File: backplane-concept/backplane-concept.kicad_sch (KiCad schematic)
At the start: 2 parts

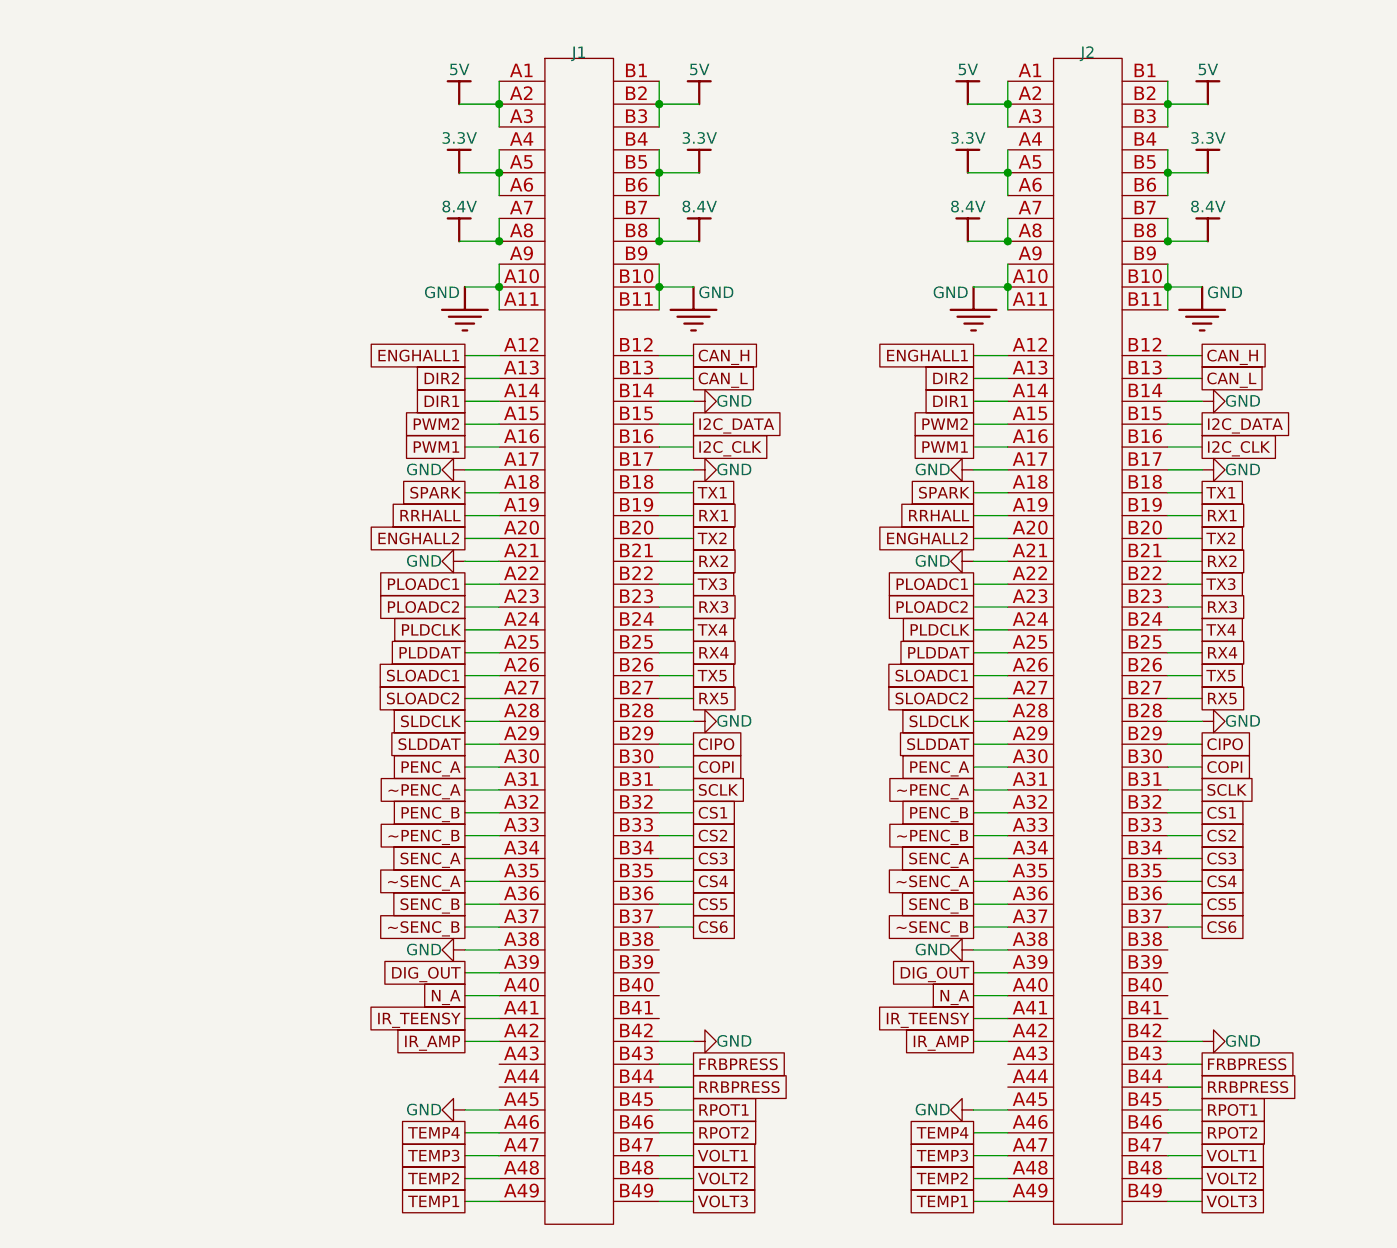
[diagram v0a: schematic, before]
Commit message: Rev
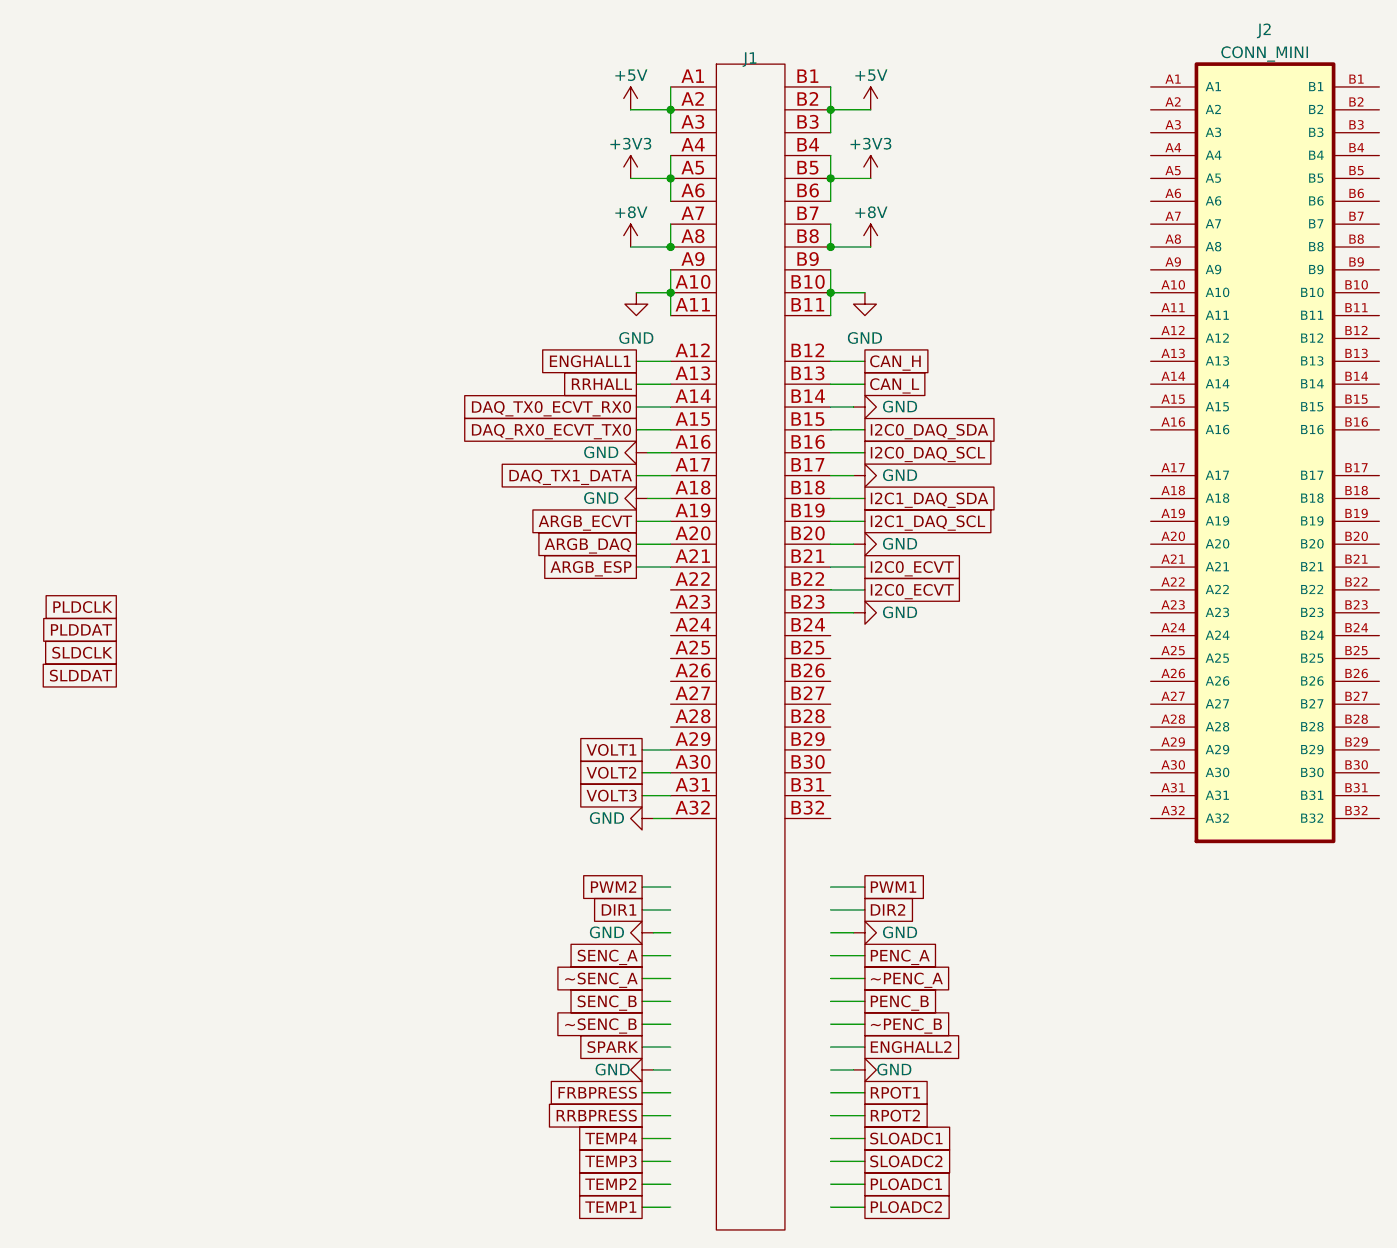
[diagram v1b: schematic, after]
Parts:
- removed J2: ~, !footprints:9-1734774-5, symbol 9-1734774-5:PCIE
- added J2: CONN_MINI, CONN_10018784-10201TLF, symbol 10018784-10201TLF:10018784-10201TLF
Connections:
- net RX3 is gone; now on net GND: J1.B23
- net TX2 is gone; now on net GND: J1.B20
- net TX3 is gone; now on net I2C0_ECVT: J1.B22
- net DIR1: no longer J1.A14
- net DIR2: no longer J1.A13
- net ENGHALL2: no longer J1.A20
- net FRBPRESS: no longer J1.B43
- net GND: now also J1.A16, J1.A18, J1.A32; no longer J1.A17, J1.A21, J1.A38, J1.A45, J1.B28, J1.B42
- net PENC_A: no longer J1.A30
- net PENC_B: no longer J1.A32
- net PLDCLK: no longer J1.A24
- net PLDDAT: no longer J1.A25
- net PLOADC1: no longer J1.A22
- net PLOADC2: no longer J1.A23
- net PWM1: no longer J1.A16
- net PWM2: no longer J1.A15
- net RPOT1: no longer J1.B45
- net RPOT2: no longer J1.B46
- net RRBPRESS: no longer J1.B44
- net RRHALL: now also J1.A13; no longer J1.A19
- net SENC_A: no longer J1.A34
- net SENC_B: no longer J1.A36
- net SLDCLK: no longer J1.A28
- net SLDDAT: no longer J1.A29
- net SLOADC1: no longer J1.A26
- net SLOADC2: no longer J1.A27
- net SPARK: no longer J1.A18
- net TEMP1: no longer J1.A49
- net TEMP2: no longer J1.A48
- net TEMP3: no longer J1.A47
- net TEMP4: no longer J1.A46
- net VOLT1: now also J1.A29; no longer J1.B47
- net VOLT2: now also J1.A30; no longer J1.B48
- net VOLT3: now also J1.A31; no longer J1.B49
- net ~PENC_A: no longer J1.A31
- net ~PENC_B: no longer J1.A33
- net ~SENC_A: no longer J1.A35
- net ~SENC_B: no longer J1.A37
- net 3.3V renamed +3V3
- net 5V renamed +5V
- net 8.4V renamed +8V
- net CIPO: no longer names the net of J1.B29
- net COPI: no longer names the net of J1.B30
- net CS1: no longer names the net of J1.B32
- removed net CS2: J1.B33
- removed net CS3: J1.B34
- removed net CS4: J1.B35
- removed net CS5: J1.B36
- removed net CS6: J1.B37
- removed net DIG_OUT: J1.A39
- net I2C_CLK renamed I2C0_DAQ_SCL
- net I2C_DATA renamed I2C0_DAQ_SDA
- removed net IR_AMP: J1.A42
- removed net IR_TEENSY: J1.A41
- removed net N_A: J1.A40
- net RX1 renamed I2C1_DAQ_SCL
- net RX2 renamed I2C0_ECVT
- net RX4: no longer names the net of J1.B25
- net RX5: no longer names the net of J1.B27
- net SCLK: no longer names the net of J1.B31
- net TX1 renamed I2C1_DAQ_SDA
- net TX4: no longer names the net of J1.B24
- net TX5: no longer names the net of J1.B26
- new net ARGB_DAQ: J1.A20
- new net ARGB_ECVT: J1.A19
- new net ARGB_ESP: J1.A21
- new net DAQ_RX0_ECVT_TX0: J1.A15
- new net DAQ_TX0_ECVT_RX0: J1.A14
- new net DAQ_TX1_DATA: J1.A17

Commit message: Backplane Ideas
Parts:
- removed J1: ~, !footprints:9-1734774-5, symbol 9-1734774-5:PCIE
- removed J2: CONN_MINI, CONN_10018784-10201TLF, symbol 10018784-10201TLF:10018784-10201TLF
- added J1: 6473427-1, 64734271, symbol 6473427-1:6473427-1
- added J2, J3, J4: PCIE_8x_Labeled, !footprints:9-1734774-5, symbol !CUSTOM:PCIE_8x_Labeled
- added J5, J6, J7, J8: CONN_MINI, !footprints:10018784-10200TLF, symbol !CUSTOM:PCIE_2x_Labeled
- added U4: ATA6561-GBQW-N, VDFN8_3X3_MCH, symbol ATA6561:ATA6561-GBQW-N
- added U5: ESP32-PICO-D4, Package_DFN_QFN:QFN-48-1EP_7x7mm_P0.5mm_EP5.3x5.3mm, symbol RF_Module:ESP32-PICO-D4
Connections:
- net +3V3: now also J1.B10, J1.B25, J1.B26, J2.A4 (+3V3), J2.A5 (+3V3), J2.A6 (+3V3), J2.B4 (+3V3), J2.B5 (+3V3), J2.B6 (+3V3), J3.A4 (+3V3), J3.A5 (+3V3), J3.A6 (+3V3), J3.B4 (+3V3), J3.B5 (+3V3), J3.B6 (+3V3), J4.A4 (+3V3), J4.A5 (+3V3), J4.A6 (+3V3), J4.B4 (+3V3), J4.B5 (+3V3), J4.B6 (+3V3), J5.A4 (+3V3), J5.A5 (+3V3), J5.A6 (+3V3), J5.B4 (+3V3), J5.B5 (+3V3), J5.B6 (+3V3), J6.A4 (+3V3), J6.A5 (+3V3), J6.A6 (+3V3), J6.B4 (+3V3), J6.B5 (+3V3), J6.B6 (+3V3), J7.A4 (+3V3), J7.A5 (+3V3), J7.A6 (+3V3), J7.B4 (+3V3), J7.B5 (+3V3), J7.B6 (+3V3), J8.A4 (+3V3), J8.A5 (+3V3), J8.A6 (+3V3), J8.B4 (+3V3), J8.B5 (+3V3), J8.B6 (+3V3)
- net +5V: now also J1.A1, J1.A10, J1.A18, J1.A26, J2.A1 (+5V), J2.A2 (+5V), J2.A3 (+5V), J2.B1 (+5V), J2.B2 (+5V), J2.B3 (+5V), J3.A1 (+5V), J3.A2 (+5V), J3.A3 (+5V), J3.B1 (+5V), J3.B2 (+5V), J3.B3 (+5V), J4.A1 (+5V), J4.A2 (+5V), J4.A3 (+5V), J4.B1 (+5V), J4.B2 (+5V), J4.B3 (+5V), J5.A1 (+5V), J5.A2 (+5V), J5.A3 (+5V), J5.B1 (+5V), J5.B2 (+5V), J5.B3 (+5V), J6.A1 (+5V), J6.A2 (+5V), J6.A3 (+5V), J6.B1 (+5V), J6.B2 (+5V), J6.B3 (+5V), J7.A1 (+5V), J7.A2 (+5V), J7.A3 (+5V), J7.B1 (+5V), J7.B2 (+5V), J7.B3 (+5V), J8.A1 (+5V), J8.A2 (+5V), J8.A3 (+5V), J8.B1 (+5V), J8.B2 (+5V), J8.B3 (+5V)
- net +8V: now also J1.B5, J1.B6, J2.A7 (VBATT), J2.A8 (VBATT), J2.B7 (VBATT), J2.B8 (VBATT), J3.A7 (VBATT), J3.A8 (VBATT), J3.B7 (VBATT), J3.B8 (VBATT), J4.A7 (VBATT), J4.A8 (VBATT), J4.B7 (VBATT), J4.B8 (VBATT), J5.A7 (VBATT), J5.A8 (VBATT), J5.B7 (VBATT), J5.B8 (VBATT), J6.A7 (VBATT), J6.A8 (VBATT), J6.B7 (VBATT), J6.B8 (VBATT), J7.A7 (VBATT), J7.A8 (VBATT), J7.B7 (VBATT), J7.B8 (VBATT), J8.A7 (VBATT), J8.A8 (VBATT), J8.B7 (VBATT), J8.B8 (VBATT)
- net CAN_H: now also J2.B12 (CAN_H), J3.B12 (CAN_H), J4.B12 (CAN_H), J5.B12 (CAN_H), J6.B12 (CAN_H), J7.B12 (CAN_H), J8.B12 (CAN_H)
- net CAN_L: now also J2.B13 (CAN_L), J3.B13 (CAN_L), J4.B13 (CAN_L), J5.B13 (CAN_L), J6.B13 (CAN_L), J7.B13 (CAN_L), J8.B13 (CAN_L)
- net DAQ_RX0_ECVT_TX0: now also J2.A13 (DAQ_RX0_ECVT_TX0), J3.A13 (DAQ_RX0_ECVT_TX0), J4.A13 (DAQ_RX0_ECVT_TX0), J5.A13 (DAQ_RX0_ECVT_TX0), J6.A13 (DAQ_RX0_ECVT_TX0), J7.A13 (DAQ_RX0_ECVT_TX0), J8.A13 (DAQ_RX0_ECVT_TX0)
- net DAQ_TX0_ECVT_RX0: now also J2.A12 (DAQ_TX0_ECVT_RX0), J3.A12 (DAQ_TX0_ECVT_RX0), J4.A12 (DAQ_TX0_ECVT_RX0), J5.A12 (DAQ_TX0_ECVT_RX0), J6.A12 (DAQ_TX0_ECVT_RX0), J7.A12 (DAQ_TX0_ECVT_RX0), J8.A12 (DAQ_TX0_ECVT_RX0)
- net DAQ_TX1_DATA: now also J2.A14 (DAQ_TX1_DATA), J3.A14 (DAQ_TX1_DATA), J4.A14 (DAQ_TX1_DATA), J5.A14 (DAQ_TX1_DATA), J6.A14 (DAQ_TX1_DATA), J7.A14 (DAQ_TX1_DATA), J8.A14 (DAQ_TX1_DATA)
- net GND: now also J1.A17, J1.A25, J1.A30, J1.A5, J1.B1, J1.B11, J1.B12, J1.B15, J1.B19, J1.B2, J1.B23, J1.B24, J1.B7, J2.A10 (GND), J2.A11 (GND), J2.A15 (GND), J2.A18 (GND), J2.A28 (GND), J2.A35 (GND), J2.A43 (GND), J2.A9 (GND), J2.B10 (GND), J2.B11 (GND), J2.B18 (GND), J2.B32 (GND), J2.B42 (GND), J2.B43 (GND), J2.B9 (GND), J3.A10 (GND), J3.A11 (GND), J3.A15 (GND), J3.A18 (GND), J3.A28 (GND), J3.A35 (GND), J3.A43 (GND), J3.A9 (GND), J3.B10 (GND), J3.B11 (GND), J3.B18 (GND), J3.B32 (GND), J3.B42 (GND), J3.B43 (GND), J3.B9 (GND), J4.A10 (GND), J4.A11 (GND), J4.A15 (GND), J4.A18 (GND), J4.A28 (GND), J4.A35 (GND), J4.A43 (GND), J4.A9 (GND), J4.B10 (GND), J4.B11 (GND), J4.B18 (GND), J4.B32 (GND), J4.B42 (GND), J4.B43 (GND), J4.B9 (GND), J5.A10 (GND), J5.A11 (GND), J5.A15 (GND), J5.A18 (GND), J5.A9 (GND), J5.B10 (GND), J5.B11 (GND), J5.B18 (GND), J5.B9 (GND), J6.A10 (GND), J6.A11 (GND), J6.A15 (GND), J6.A18 (GND), J6.A9 (GND), J6.B10 (GND), J6.B11 (GND), J6.B18 (GND), J6.B9 (GND), J7.A10 (GND), J7.A11 (GND), J7.A15 (GND), J7.A18 (GND), J7.A9 (GND), J7.B10 (GND), J7.B11 (GND), J7.B18 (GND), J7.B9 (GND), J8.A10 (GND), J8.A11 (GND), J8.A15 (GND), J8.A18 (GND), J8.A9 (GND), J8.B10 (GND), J8.B11 (GND), J8.B18 (GND), J8.B9 (GND)
- net I2C0_DAQ_SCL: now also J2.B15 (I2C0_DAQ_SCL), J3.B15 (I2C0_DAQ_SCL), J4.B15 (I2C0_DAQ_SCL), J5.B15 (I2C0_DAQ_SCL), J6.B15 (I2C0_DAQ_SCL), J7.B15 (I2C0_DAQ_SCL), J8.B15 (I2C0_DAQ_SCL)
- net I2C0_DAQ_SDA: now also J2.B14 (I2C0_DAQ_SDA), J3.B14 (I2C0_DAQ_SDA), J4.B14 (I2C0_DAQ_SDA), J5.B14 (I2C0_DAQ_SDA), J6.B14 (I2C0_DAQ_SDA), J7.B14 (I2C0_DAQ_SDA), J8.B14 (I2C0_DAQ_SDA)
- net I2C1_DAQ_SCL: now also J2.A17 (I2C1_DAQ_SCL), J3.A17 (I2C1_DAQ_SCL), J4.A17 (I2C1_DAQ_SCL), J5.A17 (I2C1_DAQ_SCL), J6.A17 (I2C1_DAQ_SCL), J7.A17 (I2C1_DAQ_SCL), J8.A17 (I2C1_DAQ_SCL)
- net I2C1_DAQ_SDA: now also J2.A16 (I2C1_DAQ_SDA), J3.A16 (I2C1_DAQ_SDA), J4.A16 (I2C1_DAQ_SDA), J5.A16 (I2C1_DAQ_SDA), J6.A16 (I2C1_DAQ_SDA), J7.A16 (I2C1_DAQ_SDA), J8.A16 (I2C1_DAQ_SDA)
- net RPOT1: now also J2.B46 (RPOT1), J3.B46 (RPOT1), J4.B46 (RPOT1)
- net RPOT2: now also J2.B47 (RPOT2), J3.B47 (RPOT2), J4.B47 (RPOT2)
- net SPARK: now also J2.A42 (SPARK), J3.A42 (SPARK), J4.A42 (SPARK)
- new net: U5.1 (VDDA), U5.43 (VDDA), U5.46 (VDDA)
- new net: U5.3 (VDDA3P3), U5.4 (VDDA3P3)
- new net: J2.A19, J3.A19, J4.A19
- new net: J2.A20, J3.A20, J4.A20
- new net: J2.A21, J3.A21, J4.A21
- new net: J2.A22, J3.A22, J4.A22
- new net: J2.A23, J3.A23, J4.A23
- new net: J2.A24, J3.A24, J4.A24
- new net: J2.A25, J3.A25, J4.A25
- new net: J2.A26, J3.A26, J4.A26
- new net: J2.A27, J3.A27, J4.A27
- new net: J2.B19, J3.B19, J4.B19
- new net: J2.B20, J3.B20, J4.B20
- new net: J2.B21, J3.B21, J4.B21
- new net: J2.B22, J3.B22, J4.B22
- new net: J2.B23, J3.B23, J4.B23
- new net: J2.B24, J3.B24, J4.B24
- new net: J2.B25, J3.B25, J4.B25
- new net: J2.B26, J3.B26, J4.B26
- new net: J2.B27, J3.B27, J4.B27
- new net: J2.B48, J3.B48, J4.B48
- new net: J2.B49, J3.B49, J4.B49
- new net AVDD_P: J1.B18
- new net AVDD_S: J1.B22
- new net BP_FRONT: J2.B44 (BP_FRONT), J3.B44 (BP_FRONT), J4.B44 (BP_FRONT)
- new net BP_REAR: J2.B45 (BP_REAR), J3.B45 (BP_REAR), J4.B45 (BP_REAR)
- new net DIR_P: J2.B36 (DIR_P), J3.B36 (DIR_P), J4.B36 (DIR_P)
- new net DIR_S: J2.B38 (DIR_S), J3.B38 (DIR_S), J4.B38 (DIR_S)
- new net ENCA_P: J1.A11, J2.A29 (ENCA_P), J3.A29 (ENCA_P), J4.A29 (ENCA_P)
- new net ENCA_S: J1.A19, J2.A36 (ENCA_S), J3.A36 (ENCA_S), J4.A36 (ENCA_S)
- new net ENCB_P: J1.A13, J2.A31 (ENCB_P), J3.A31 (ENCB_P), J4.A31 (ENCB_P)
- new net ENCB_S: J1.A21, J2.A38 (ENCB_S), J3.A38 (ENCB_S), J4.A38 (ENCB_S)
- new net ENCI_P: J1.A15, J2.A33 (ENCI_P), J3.A33 (ENCI_P), J4.A33 (ENCI_P)
- new net ENCI_S: J1.A23, J2.A40 (ENCI_S), J3.A40 (ENCI_S), J4.A40 (ENCI_S)
- new net HALL1_P: J1.A2
- new net HALL1_S: J1.A27
- new net HALL2_P: J1.A3
- new net HALL2_S: J1.A28
- new net HALL3_P: J1.A4
- new net HALL3_S: J1.A29
- new net HALL_ENG1: J1.B3, J2.B33 (HALL_ENG1), J3.B33 (HALL_ENG1), J4.B33 (HALL_ENG1)
- new net HALL_ENG2: J1.B4, J2.B41 (HALL_ENG2), J3.B41 (HALL_ENG2), J4.B41 (HALL_ENG2)
- new net HALL_RW: J2.B34 (HALL_RW), J3.B34 (HALL_RW), J4.B34 (HALL_RW)
- new net I2C0_ECVT_SCL: J2.B17 (I2C0_ECVT_SCL), J3.B17 (I2C0_ECVT_SCL), J4.B17 (I2C0_ECVT_SCL), J5.B17 (I2C0_ECVT_SCL), J6.B17 (I2C0_ECVT_SCL), J7.B17 (I2C0_ECVT_SCL), J8.B17 (I2C0_ECVT_SCL)
- new net I2C0_ECVT_SDA: J2.B16 (I2C0_ECVT_SDA), J3.B16 (I2C0_ECVT_SDA), J4.B16 (I2C0_ECVT_SDA), J5.B16 (I2C0_ECVT_SDA), J6.B16 (I2C0_ECVT_SDA), J7.B16 (I2C0_ECVT_SDA), J8.B16 (I2C0_ECVT_SDA)
- new net I2C1_ECVT_EXT_SCL: J1.B9, J2.B40 (I2C1_ECVT_EXT_SCL), J3.B40 (I2C1_ECVT_EXT_SCL), J4.B40 (I2C1_ECVT_EXT_SCL)
- new net I2C1_ECVT_EXT_SDA: J1.B8, J2.B39 (I2C1_ECVT_EXT_SDA), J3.B39 (I2C1_ECVT_EXT_SDA), J4.B39 (I2C1_ECVT_EXT_SDA)
- new net IN+_P: J1.B16
- new net IN+_S: J1.B20
- new net IN-_P: J1.B17
- new net IN-_S: J1.B21
- new net LOADC_CLK_P: J2.B28 (LOADC_CLK_P), J2.B30 (LOADC_CLK_S), J3.B28 (LOADC_CLK_P), J3.B30 (LOADC_CLK_S), J4.B28 (LOADC_CLK_P), J4.B30 (LOADC_CLK_S)
- new net LOADC_DAT_P: J2.B29 (LOADC_DAT_P), J3.B29 (LOADC_DAT_P), J4.B29 (LOADC_DAT_P)
- new net LOADC_DAT_S: J2.B31 (LOADC_DAT_S), J3.B31 (LOADC_DAT_S), J4.B31 (LOADC_DAT_S)
- new net MOT1_P: J1.A7
- new net MOT1_S: J1.A32
- new net MOT2_P: J1.A8
- new net MOT2_S: J1.A33
- new net MOT3_P: J1.A9
- new net MOT3_S: J1.A34
- new net PWM_P: J2.B35 (PWM_P), J3.B35 (PWM_P), J4.B35 (PWM_P)
- new net PWM_S: J2.B37 (PWM_S), J3.B37 (PWM_S), J4.B37 (PWM_S)
- new net THERM_A1_CASE: J1.B13, J2.A46 (THERM_A1_CASE), J3.A46 (THERM_A1_CASE), J4.A46 (THERM_A1_CASE)
- new net THERM_A2_CASE: J1.B14, J2.A47 (THERM_A2_CASE), J3.A47 (THERM_A2_CASE), J4.A47 (THERM_A2_CASE)
- new net THERM_A3: J2.A48 (THERM_A3), J3.A48 (THERM_A3), J4.A48 (THERM_A3)
- new net THERM_A4: J2.A49 (THERM_A4), J3.A49 (THERM_A4), J4.A49 (THERM_A4)
- new net THERM_P: J1.A6, J2.A44 (THERM_P), J3.A44 (THERM_P), J4.A44 (THERM_P)
- new net THERM_S: J1.A31, J2.A45 (THERM_S), J3.A45 (THERM_S), J4.A45 (THERM_S)
- new net ~ENCA_P: J1.A12, J2.A30 (~ENCA_P), J3.A30 (~ENCA_P), J4.A30 (~ENCA_P)
- new net ~ENCA_S: J1.A20, J2.A37 (~ENCA_S), J3.A37 (~ENCA_S), J4.A37 (~ENCA_S)
- new net ~ENCB_P: J1.A14, J2.A32 (~ENCB_P), J3.A32 (~ENCB_P), J4.A32 (~ENCB_P)
- new net ~ENCB_S: J1.A22, J2.A39 (~ENCB_S), J3.A39 (~ENCB_S), J4.A39 (~ENCB_S)
- new net ~ENCI_P: J1.A16, J2.A34 (~ENCI_P), J3.A34 (~ENCI_P), J4.A34 (~ENCI_P)
- new net ~ENCI_S: J1.A24, J2.A41 (~ENCI_S), J3.A41 (~ENCI_S), J4.A41 (~ENCI_S)
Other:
- added sheet Analog Frontend (analog_frontend.kicad_sch)
